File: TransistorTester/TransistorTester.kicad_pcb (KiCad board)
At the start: 2 copper layers, 50 x 29 mm, 19 parts, among them J1 Conn_01x02, J10 Conn_01x03_Pin, J2 Conn_01x02, J3 Conn_01x02, J4 Conn_01x03_Pin, J5 Conn_01x03_Pin, J6 Conn_01x03_Pin, J7 Conn_01x02, J8 Conn_01x03_Pin, J9 Conn_01x03_Pin

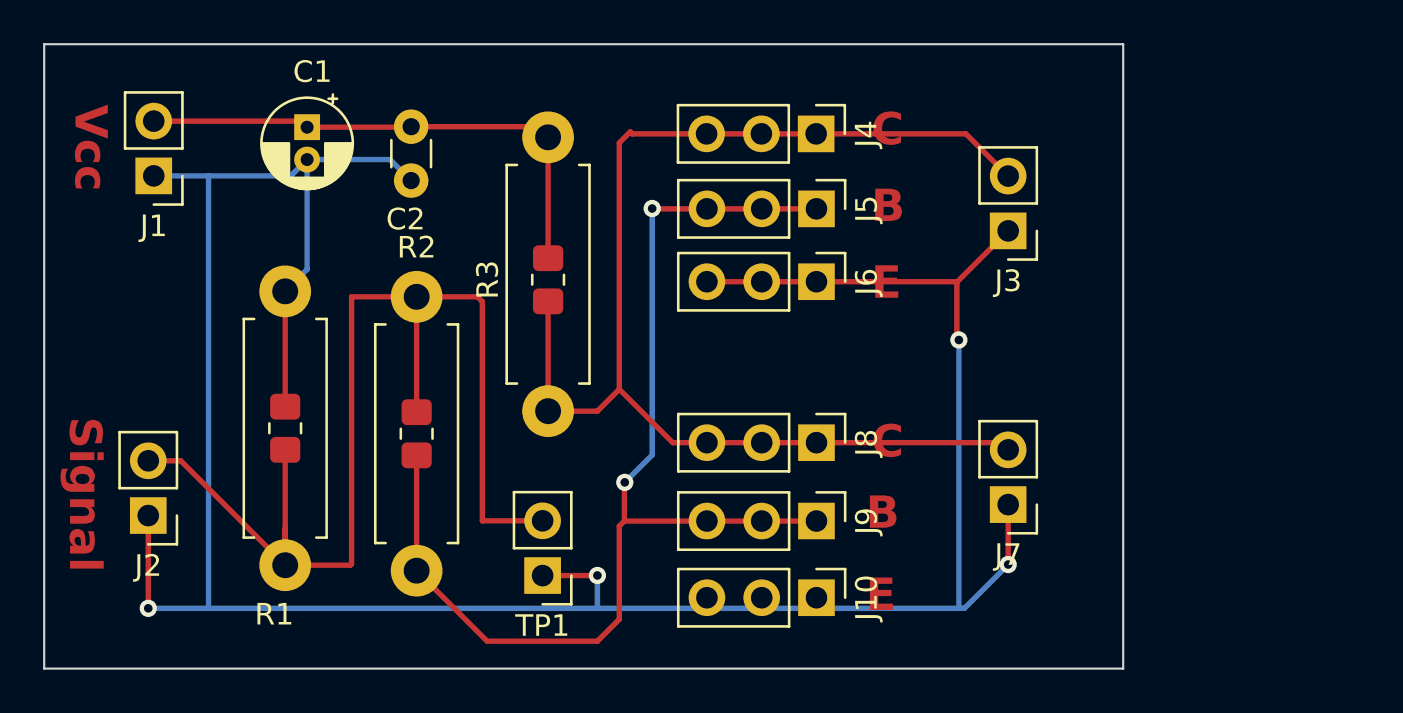
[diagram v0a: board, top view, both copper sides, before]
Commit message: fix resistors
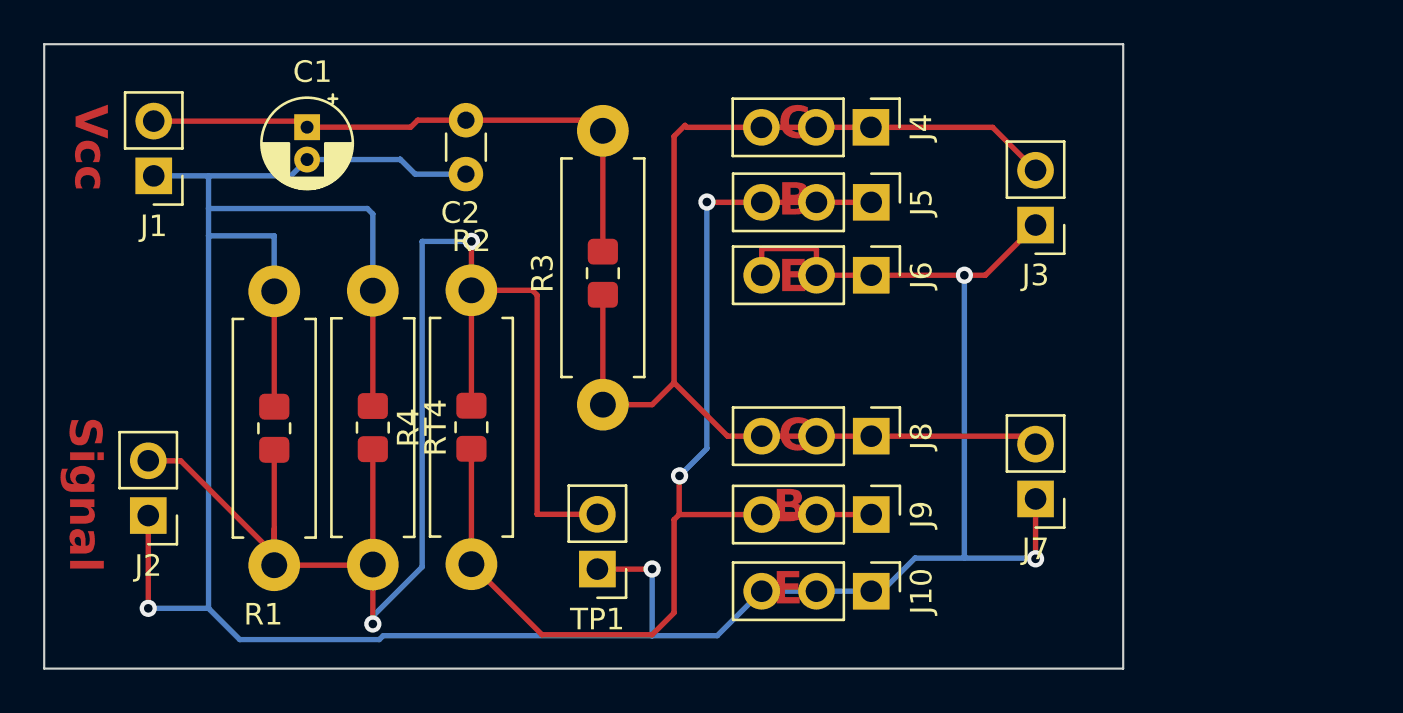
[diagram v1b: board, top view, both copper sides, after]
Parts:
- added R4: 100, Resistor_SMD:R_0805_2012Metric_Pad1.20x1.40mm_HandSolder, F.Cu at (66.0, 68.6)
- added RT4: 100, Resistor_THT:R_Axial_DIN0411_L9.9mm_D3.6mm_P12.70mm_Horizontal, F.Cu at (66.0, 62.2)
- R1: value 50R -> 100
- RT1: value 50 -> 100
- moved C2 2.56 mm to (70.4, 56.8)
- moved R2 2.56 mm to (70.6, 68.6)
- moved J10 2.56 mm to (89.2, 76.2)
- moved J4 2.56 mm to (89.1, 54.7)
- moved J5 2.56 mm to (89.2, 58.1)
- moved J6 2.56 mm to (89.2, 61.5)
- moved J8 2.56 mm to (89.2, 69.0)
- moved J9 2.56 mm to (89.2, 72.6)
- moved R3 2.56 mm to (76.7, 61.4)
- moved RT2 2.56 mm to (70.6, 74.9)
- moved RT3 2.56 mm to (76.7, 67.5)
- moved TP1 2.56 mm to (76.5, 75.1)
- moved J3 1.30 mm to (96.8, 59.2)
- moved J7 1.30 mm to (96.8, 71.9)
- moved R1 0.51 mm to (61.5, 68.6)
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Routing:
- net GND: track 126.6 -> 148.6 mm
- net Net-(J2-Pin_2): track 55.4 -> 72.8 mm, vias 0 -> 2
- net Net-(J1-Pin_2): track 24.3 -> 27.0 mm
- net Net-(J3-Pin_2): track 58.5 -> 56.0 mm

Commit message: adapt to board
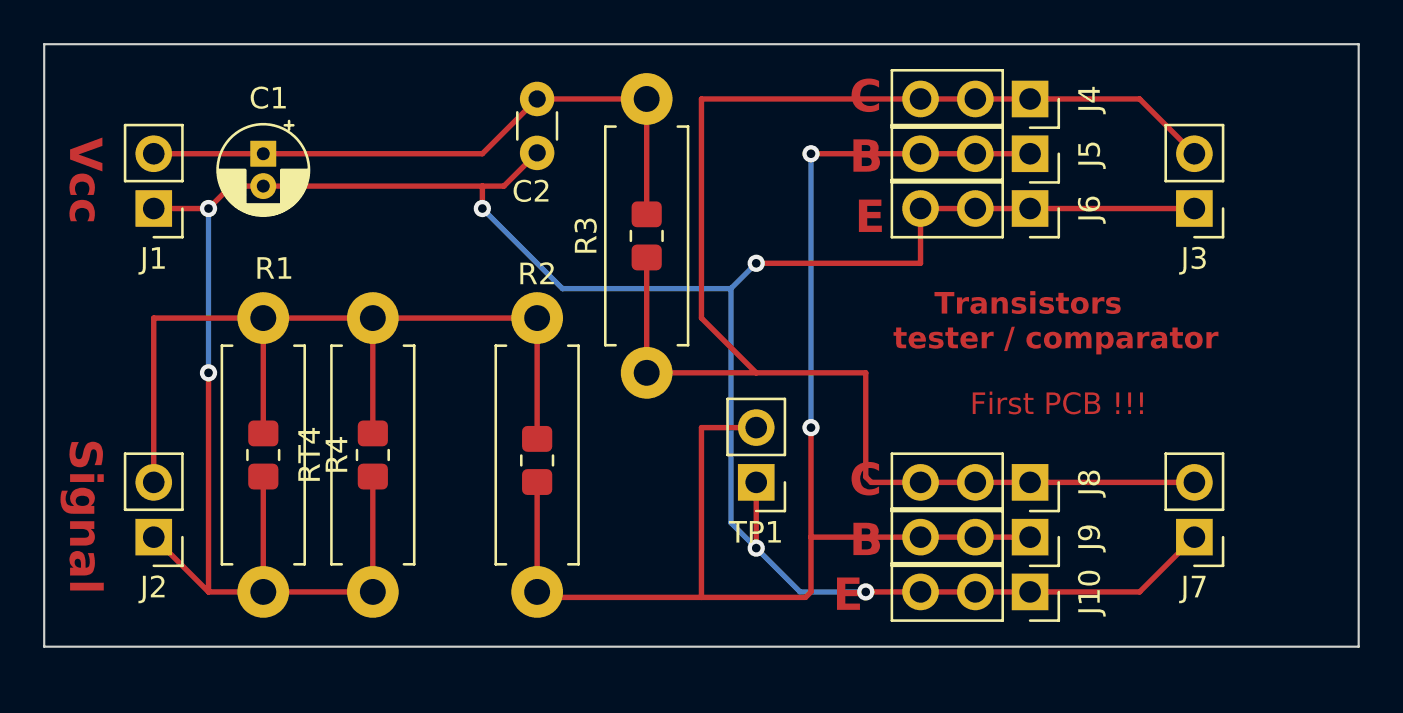
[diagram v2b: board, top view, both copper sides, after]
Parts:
- J10, J4, J5, J6, J8, J9: footprint Connector_PinHeader_2.54mm:PinHeader_1x03_P2.54mm_Vertical -> Connector_PinSocket_2.54mm:PinSocket_1x03_P2.54mm_Vertical
- moved RT4 14.0 mm to (66.0, 76.2), turned to 90 degrees
- moved RT1 13.9 mm to (61.0, 76.2), turned to 90 degrees
- moved TP1 8.39 mm to (83.8, 71.1)
- moved J6 7.99 mm to (96.5, 58.4)
- moved J5 7.70 mm to (96.5, 55.9)
- moved J8 7.67 mm to (96.5, 71.1)
- moved J7 7.58 mm to (104.1, 73.7)
- moved J4 7.50 mm to (96.5, 53.3)
- moved J9 7.44 mm to (96.5, 73.7)
- moved J3 7.41 mm to (104.1, 58.4)
- moved J10 7.37 mm to (96.5, 76.2)
- moved C2 3.45 mm to (73.7, 55.8)
- moved R2 3.41 mm to (73.7, 70.1)
- moved RT2 3.31 mm to (73.7, 76.2)
- moved R3 2.67 mm to (78.7, 59.7)
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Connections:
- TP1 pad 2: Net-(J2-Pin_2) -> Net-(J5-Pin_1)
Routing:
- net Net-(J2-Pin_2): track 72.8 -> 41.7 mm, vias 2 -> 0
- net Net-(J3-Pin_2): track 56.0 -> 73.3 mm
- net Net-(J5-Pin_1): track 52.7 -> 69.2 mm
- net GND: track 148.6 -> 134.9 mm, vias 4 -> 6
- net Net-(J1-Pin_2): track 27.0 -> 29.3 mm
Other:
- board size 50 x 29 mm -> 61 x 27.9 mm
- board text added: "First PCB !!!"
- board text added: "Transistors tester / comparator"
